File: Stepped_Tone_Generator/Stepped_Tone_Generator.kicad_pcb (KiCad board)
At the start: 2 copper layers, 50 x 34.5 mm, 20 parts, among them J1 FCV, J2 PWCV, J3 DC IN, J4 Audio Out, SW2 ON/OFF, U1 555, U2 555

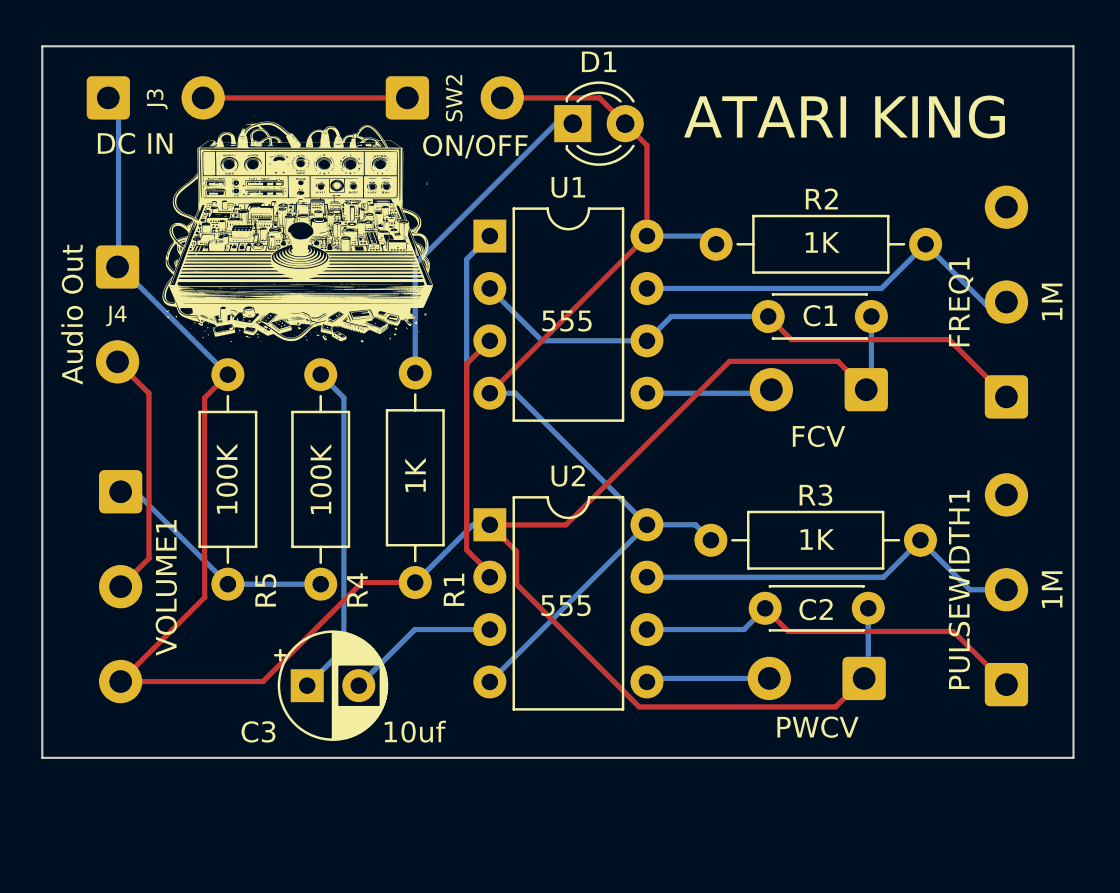
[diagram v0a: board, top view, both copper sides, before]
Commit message: atari king layouts
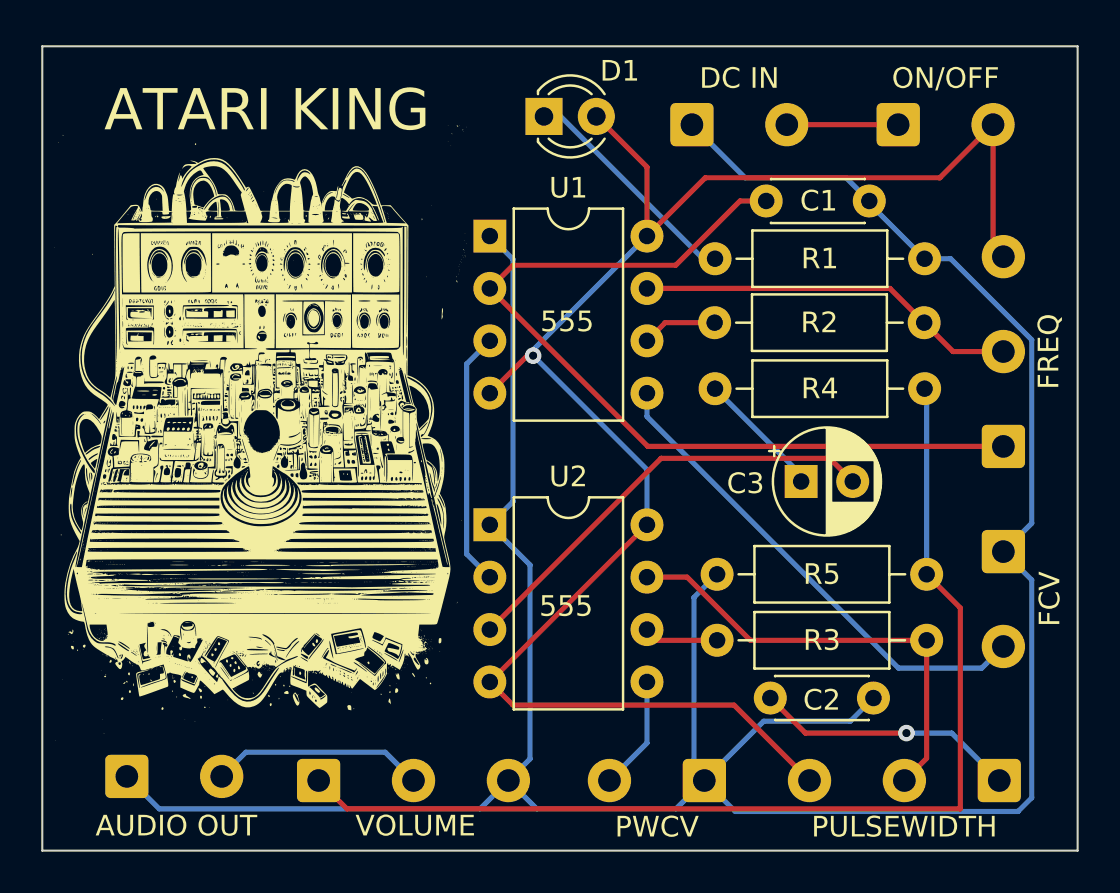
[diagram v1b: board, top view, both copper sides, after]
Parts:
- removed the G*** at (127.5, 59.0)
- added G***: LOGO, images:atari_large_long, F.Cu at (125.6, 68.8)
- AUDIO OUT: renamed from J4; value Audio Out -> AUDIO OUT
- C1: value 0.01uf -> .01uf
- C2: value 0.1uf -> .1uf
- DC IN: renamed from J3
- R4: value 100K -> 10K
- R5: value 100K -> 4.7K
- moved R1 29.3 mm to (157.8, 60.3), turned to 180 degrees
- moved DC IN 28.3 mm to (146.5, 53.8)
- moved C3 25.9 mm to (151.8, 71.1)
- moved R5 25.6 mm to (147.7, 75.6), turned to 0 degrees
- moved AUDIO OUT 24.7 mm to (119.1, 85.4), turned to 0 degrees
- moved ON/OFF 23.8 mm to (156.5, 53.8)
- moved R4 19.1 mm to (147.6, 66.6), turned to 0 degrees
- moved VOLUME 17.0 mm to (128.4, 85.6), turned to 0 degrees
- moved R3 11.0 mm to (147.7, 78.8), turned to 0 degrees
- moved R2 10.9 mm to (147.6, 63.4), turned to 0 degrees
- moved FCV 10.3 mm to (161.6, 74.5), turned to -90 degrees
- moved PWCV 9.20 mm to (147.1, 85.6)
- moved C1 5.60 mm to (155.1, 57.5)
- moved PULSEWIDTH 4.66 mm to (161.4, 85.6), turned to 180 degrees
- moved C2 4.36 mm to (155.3, 81.6)
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- renumbered J1 to FCV, FREQ1 to FREQ, SW2 to ON/OFF, PULSEWIDTH1 to PULSEWIDTH, J2 to PWCV, VOLUME1 to VOLUME
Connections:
- C2 pad 2: Net-(C2-Pad2) -> Net-(PULSEWIDTH1-Pad1)
- FREQ pad 3: unconnected-(FREQ1-Pad3) -> /PWR
- PULSEWIDTH pad 1: Net-(C2-Pad2) -> Net-(PULSEWIDTH1-Pad1)
- PULSEWIDTH pad 3: unconnected-(PULSEWIDTH1-Pad3) -> /PWR
- R2 pad 1: Net-(FREQ1-Pad2) -> Net-(U1-Pad6)
- R2 pad 2: /PWR -> Net-(FREQ1-Pad2)
- R3 pad 1: Net-(PULSEWIDTH1-Pad2) -> Net-(U2-Pad6)
- R3 pad 2: /PWR -> Net-(PULSEWIDTH1-Pad2)
- U1 pad 6: Net-(C1-Pad2) -> Net-(U1-Pad6)
- U2 pad 6: Net-(C2-Pad2) -> Net-(U2-Pad6)
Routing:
- net Net-(R4-Pad2): track 11.6 -> 52.8 mm
- net /PWR: track 51.1 -> 82.1 mm, vias 0 -> 1
- net GND: track 120.1 -> 140.4 mm
- net Net-(C2-Pad2): track 19.4 -> 0.00 mm
- net Net-(J1-PadT): track 6.10 -> 23.9 mm
- net Net-(C1-Pad2): track 28.2 -> 43.2 mm
- net Net-(C3-Pad2): track 7.48 -> 21.5 mm
- net Net-(PULSEWIDTH1-Pad1): track 0.00 -> 12.8 mm, vias 0 -> 1
- net Net-(C3-Pad1): track 16.3 -> 6.23 mm
- net Net-(D1-Pad1): track 15.7 -> 11.2 mm
- net +9V: track 9.90 -> 5.40 mm
- net Net-(U1-Pad6): track 0.00 -> 3.64 mm
- net Net-(U2-Pad6): track 0.00 -> 3.62 mm
- net Net-(PULSEWIDTH1-Pad2): track 19.2 -> 22.1 mm
- net Net-(J4-PadT): track 12.1 -> 10.4 mm
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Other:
- board size 50 x 34.5 mm -> 50.2 x 39 mm
